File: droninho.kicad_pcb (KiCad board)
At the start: 2 copper layers, 26 x 49 mm, 19 parts, among them J1 Conn_01x02_Pin, J2 M2, J3 M1, J4 M3, J5 M4, Q1 SI2300, Q2 SI2300, Q3 SI2300, Q4 SI2300, U1 ESP32 Dev Kit, U3 MPU9250/6500

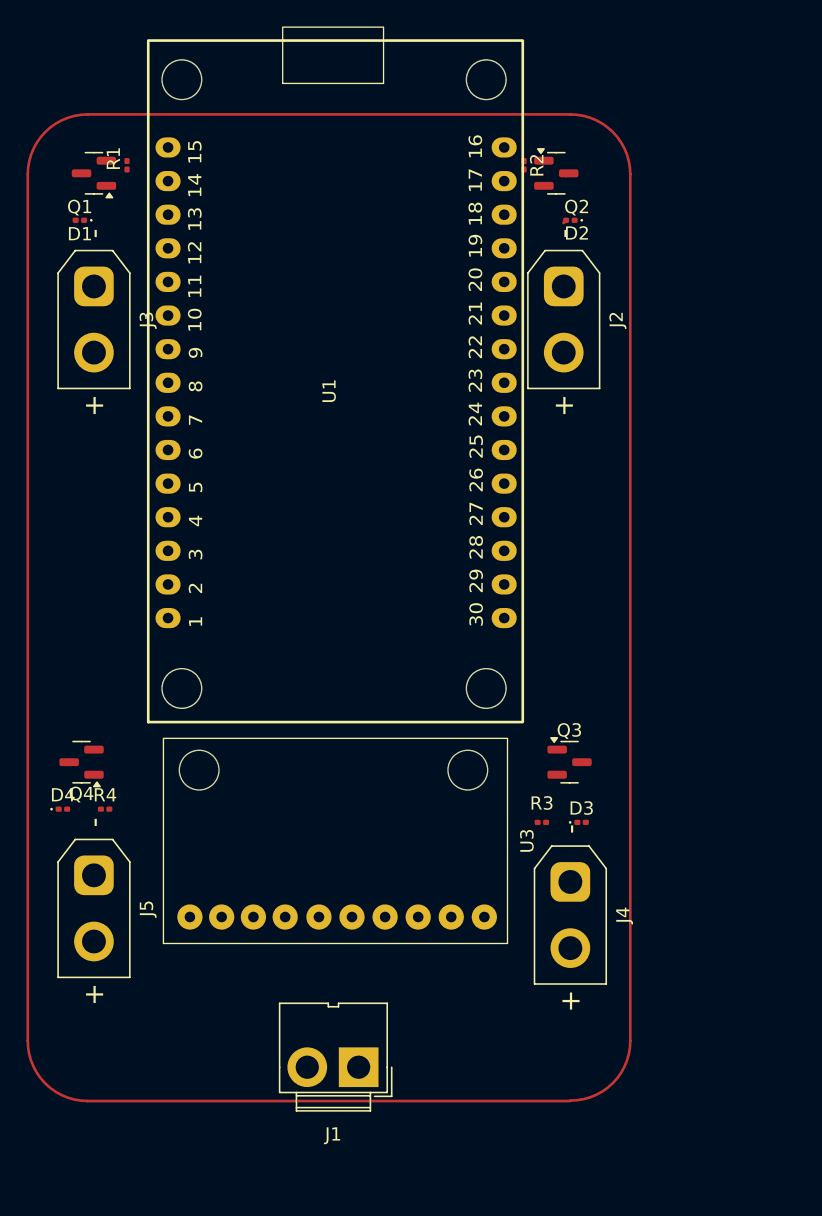
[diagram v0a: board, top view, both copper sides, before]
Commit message: PCB feito.
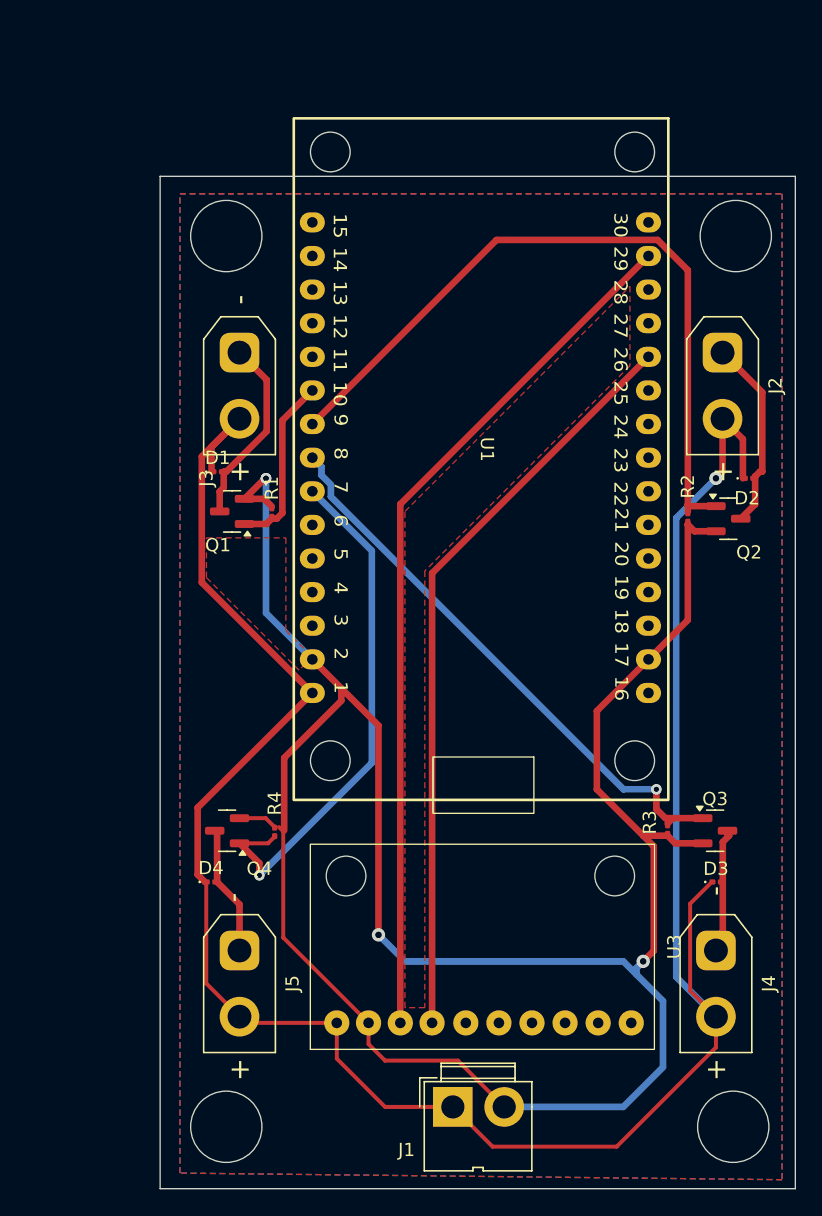
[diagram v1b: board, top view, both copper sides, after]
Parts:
- moved R2 29.4 mm to (160.9, 91.0)
- moved Q2 29.2 mm to (163.9, 91.0)
- moved R1 28.4 mm to (129.4, 90.6)
- moved Q1 27.6 mm to (126.4, 90.5)
- moved D2 23.7 mm to (165.5, 88.0), turned to 0 degrees
- moved D1 21.7 mm to (125.3, 87.5), turned to 0 degrees
- moved U3 13.7 mm to (132.3, 131.2)
- moved J2 13.0 mm to (163.5, 78.5)
- moved R4 12.9 mm to (129.7, 114.7), turned to 90 degrees
- moved U1 12.5 mm to (145.4, 86.2), turned to -90 degrees
- moved D4 12.5 mm to (124.8, 118.5)
- moved J5 12.4 mm to (127.0, 123.7)
- moved J4 12.2 mm to (163.0, 123.7)
- moved Q3 12.2 mm to (162.9, 114.6)
- moved Q4 12.2 mm to (126.1, 114.6)
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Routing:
- net GND: track 0.00 -> 178.1 mm, vias 0 -> 4
- net +3.3V: track 0.00 -> 171.3 mm, vias 0 -> 1
- net /SCL: track 0.00 -> 65.7 mm
- net /SDA: track 0.00 -> 57.1 mm
- net /PWM2: track 0.00 -> 55.5 mm
- net /PWM3: track 0.00 -> 43.1 mm, vias 0 -> 1
- net /PWM4: track 0.00 -> 40.3 mm, vias 0 -> 1
- net /M1-: track 0.00 -> 14.4 mm
- net /M2-: track 0.53 -> 14.6 mm
- net /PWM1: track 0.00 -> 13.4 mm
- net /M4-: track 0.00 -> 9.83 mm
- net /M3-: track 0.00 -> 9.52 mm
- added copper zone on B.Cu, net GND
- added copper zone on F.Cu, net GND
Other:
- board size 26 x 49 mm -> 48 x 76.5 mm
